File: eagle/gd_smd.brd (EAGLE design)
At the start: 101.9 x 165.1 mm, 86 parts, among them K1 G5V-2, X4 BU-SMA-V

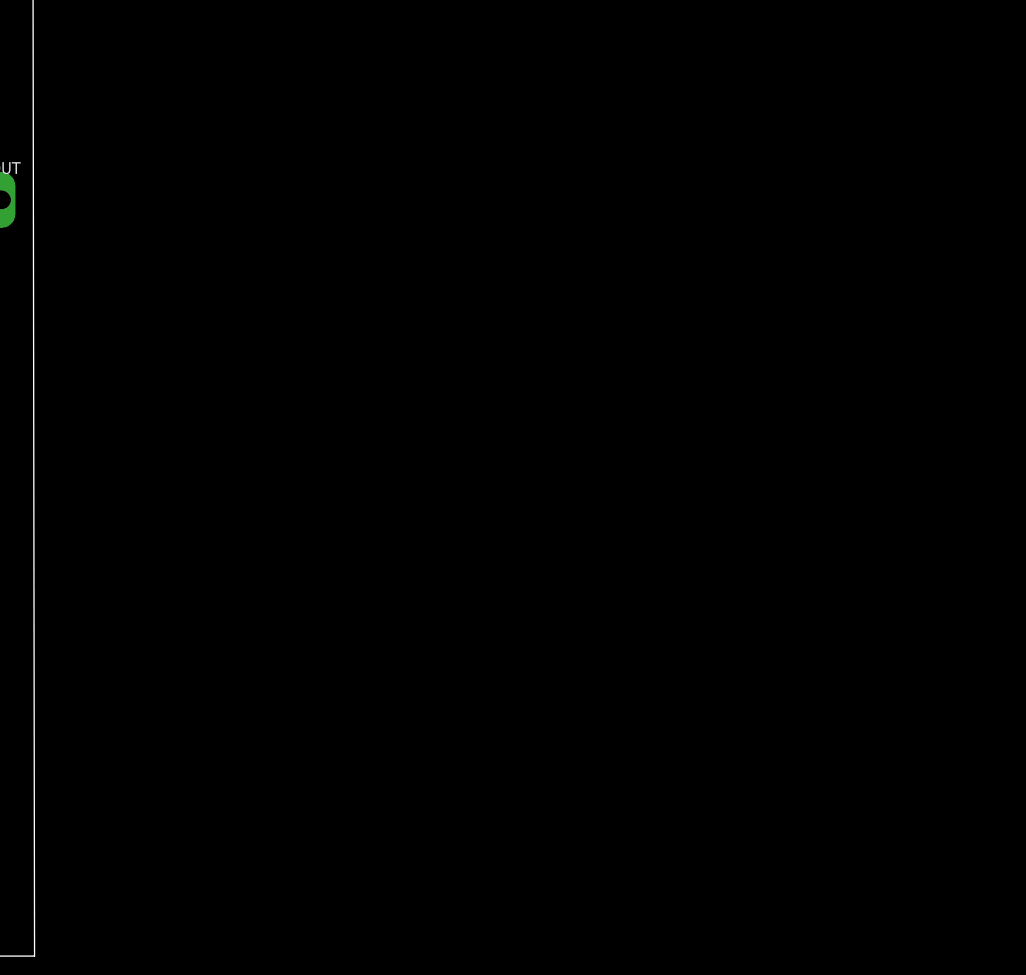
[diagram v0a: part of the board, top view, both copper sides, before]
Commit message: smd layout, debug code
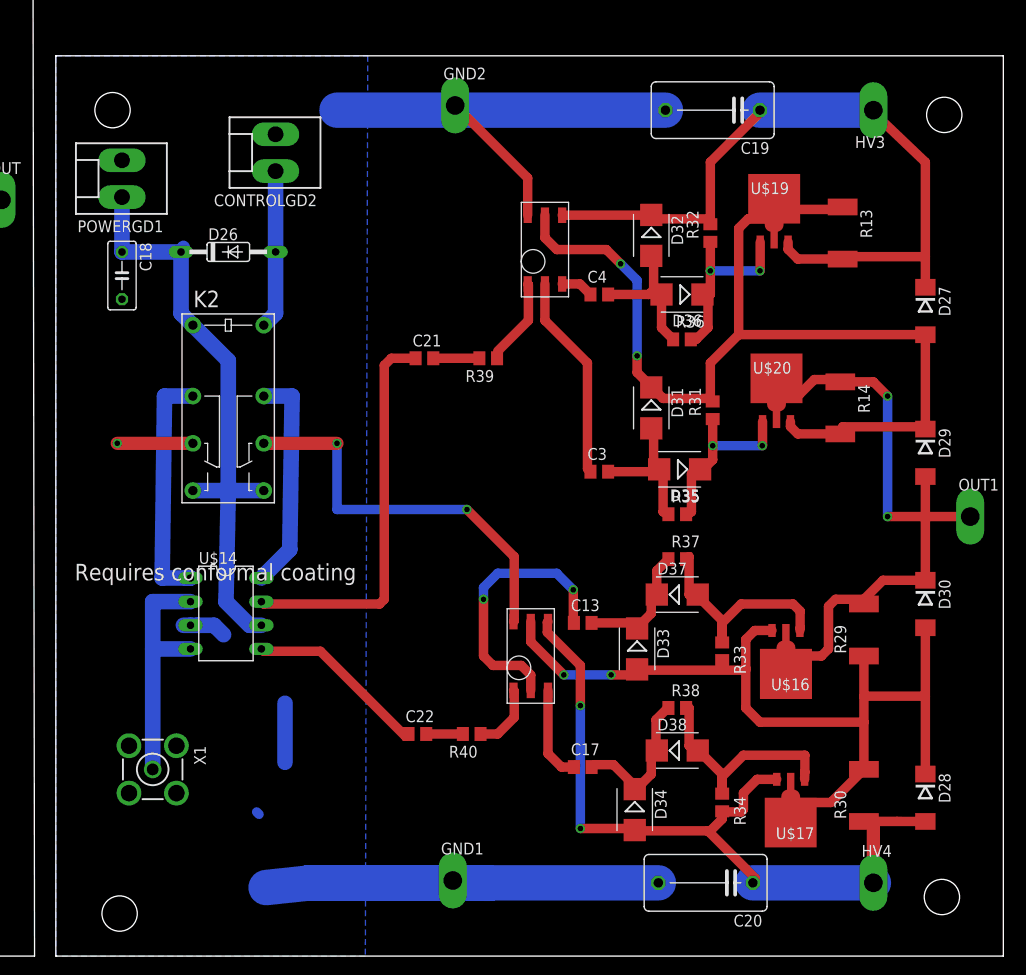
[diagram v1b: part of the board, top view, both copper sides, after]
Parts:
- added C13, C17, C21, C22, C3, C4: 1u, resistor:C0805
- added C18: 10n, rcl:C050-030X075
- added C19, C20: 10p, resistor:C102-064X133
- added CONTROLGD2, POWERGD1: (no value), con-molex:KK-156-2
- added D26: 1N4148DO35-10, diode:DO35-10
- added D27, D28, D29, D30: SMBJ170D-M3/H, diode:DO214AA
- added D31, D32, D33, D34: 1SMB5918BT3G, diode:SMB
- added D35, D36, D37, D38: (no value), diode:SMB
- added GND1, GND2, HV3, HV4, OUT1: TPPAD1-20Y, testpad:P1-20Y
- added K2: G5V-2, relay:G5V-2
- added R13, R14, R29, R30: 10M, rcl:R2512
- added R31, R32, R33, R34: 100k, rcl:R0805
- added R35, R36, R37, R38, R39, R40: 10, rcl:R0805
- added U$14: UCC27425, texas:DIL08
- added U$15, U$18: DA-2320SMD6, trafo:SMD6
- added U$16, U$17: VN2450, transistor-fet:SOT89-BCE
- added U$19, U$20: VP2450, transistor-fet:SOT89-BCE
- added X1: BU-SMA-V, con-coax:BU-SMA-V
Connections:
- new net +15V1: C18.1, D26.C, K2.1, K2.8, K2.9, POWERGD1.1, U$14.6
- new net ENSW1: CONTROLGD2.1, D26.A, K2.16
- new net GND1: C18.2, C19.2, C20.2, CONTROLGD2.2, GND1.TP, GND2.TP, K2.11, K2.6, POWERGD1.2, U$14.3, U$15.P$6, U$18.P$6, X1.2, X1.3, X1.4, X1.5
- new net N$19: K2.4, U$14.1
- new net N$20: K2.13, U$14.8
- new net N$21: C3.1, U$15.P$2
- new net N$3: U$14.2, U$14.4, X1.1
- new net N$31: C4.1, U$15.P$3
- new net N$39: C13.1, U$18.P$2
- new net N$44: C17.1, U$18.P$3
- new net N$45: C13.2, D33.C, D37.C, R37.1
- new net N$52: C17.2, D34.C, D38.C, R38.1
- new net N$53: C4.2, D32.A, D36.A, R36.1
- new net N$54: C19.1, D27.C, D32.C, HV3.TP, R13.2, R32.2, U$15.P$4, U$19.E
- new net N$55: D28.C, D30.A, D33.A, R29.1, R30.2, R33.2, U$16.E, U$17.C, U$17.C@1, U$18.P$5
- new net N$56: D27.A, D29.C, D31.C, R13.1, R14.2, R31.2, U$15.P$5, U$19.C, U$19.C@1, U$20.E
- new net N$57: D35.C, R31.1, R35.2, U$20.B
- new net N$58: C3.2, D31.A, D35.A, R35.1
- new net N$59: D38.A, R34.1, R38.2, U$17.B
- new net N$6: C21.1, U$14.7
- new net N$60: D36.C, R32.1, R36.2, U$19.B
- new net N$61: D37.A, R33.1, R37.2, U$16.B
- new net N$62: C20.1, D28.A, D34.A, HV4.TP, R30.1, R34.2, U$17.E, U$18.P$4
- new net N$63: R39.1, U$15.P$1
- new net N$64: C21.2, R39.2
- new net N$65: R40.1, U$18.P$1
- new net N$66: C22.2, R40.2
- new net N$67: D29.A, D30.C, OUT1.TP, R14.1, R29.2, U$16.C, U$16.C@1, U$20.C, U$20.C@1
- new net N$9: C22.1, U$14.5
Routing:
- net GND1: track 0.00 -> 176.2 mm, vias 0 -> 3
- net N$56: track 0.00 -> 111.9 mm, vias 0 -> 2
- net N$55: track 0.00 -> 95.4 mm, vias 0 -> 2
- net N$62: track 0.00 -> 85.0 mm, vias 0 -> 2
- net N$54: track 0.00 -> 80.6 mm
- net N$67: track 0.00 -> 67.9 mm, vias 0 -> 2
- net +15V1: track 0.00 -> 65.7 mm
- net N$6: track 0.00 -> 42.4 mm
- net N$39: track 0.00 -> 29.6 mm, vias 0 -> 2
- net N$19: track 0.00 -> 26.2 mm
- net N$3: track 0.00 -> 26.2 mm
- net N$59: track 0.00 -> 25.5 mm
- net N$61: track 0.00 -> 25.4 mm
- net N$20: track 0.00 -> 23.9 mm
- net N$21: track 0.00 -> 22.2 mm
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- added copper zone on layer 16, net GND1
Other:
- board size 101.9 x 165.1 mm -> 206 x 165.1 mm
